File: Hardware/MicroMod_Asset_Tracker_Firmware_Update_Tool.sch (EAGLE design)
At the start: 23 parts, among them J5 MICROMOD-2222, U2 CH340C

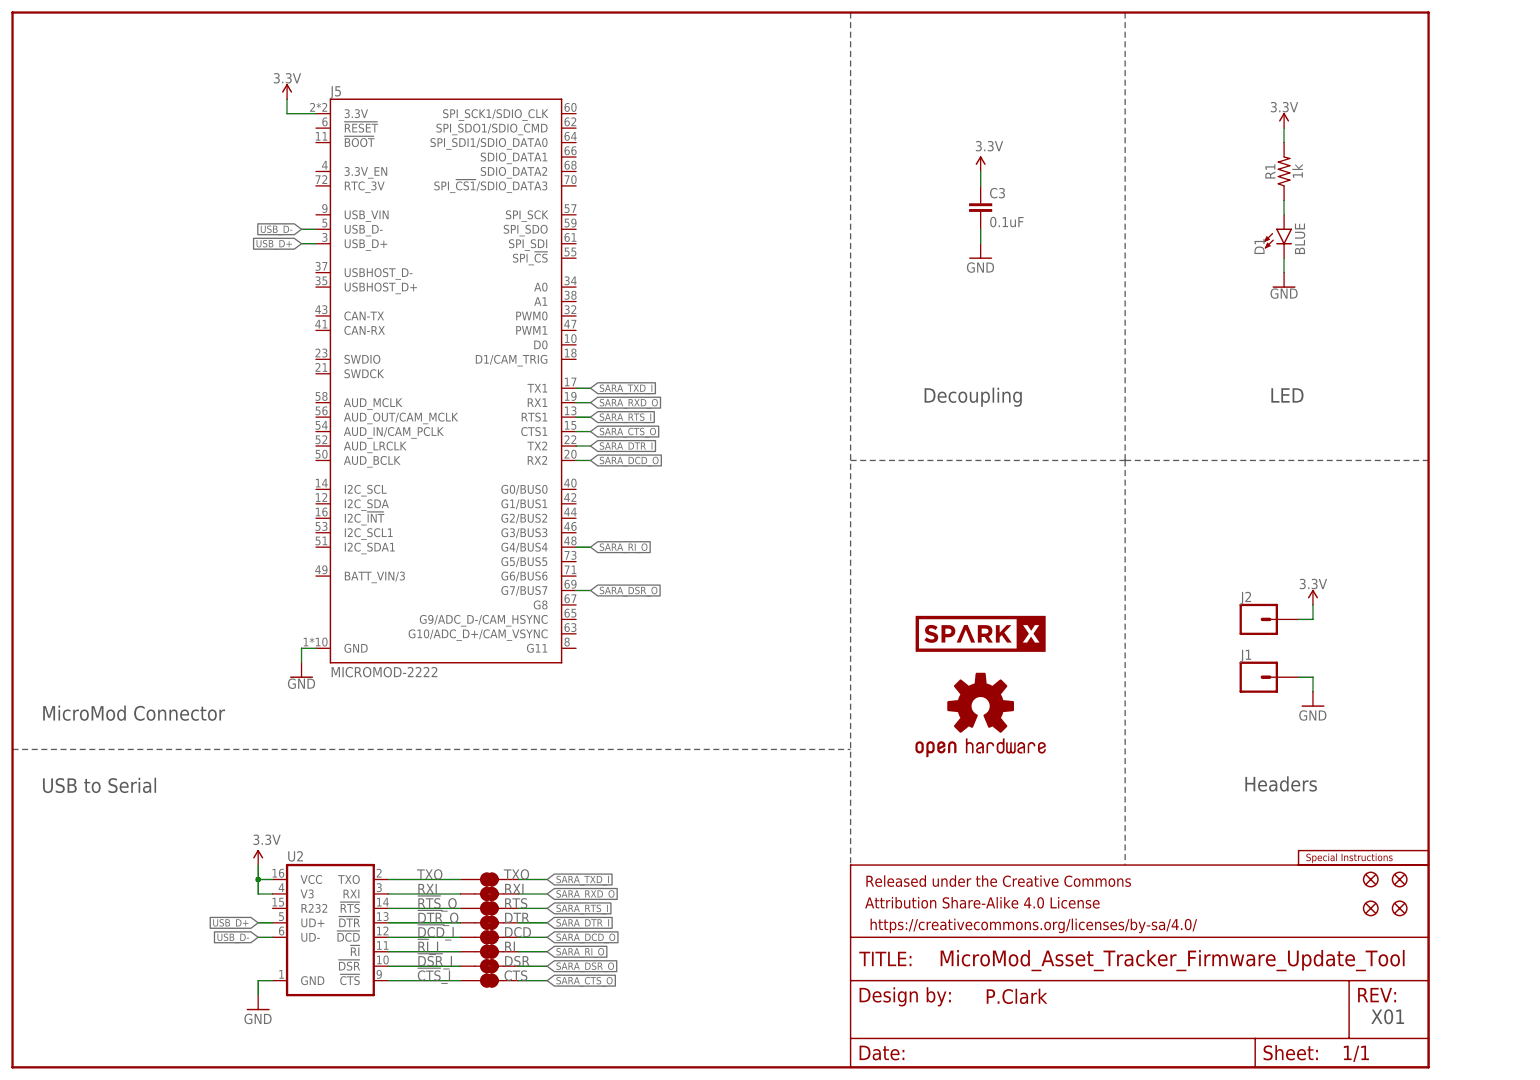
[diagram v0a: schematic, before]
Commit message: Updates for v10
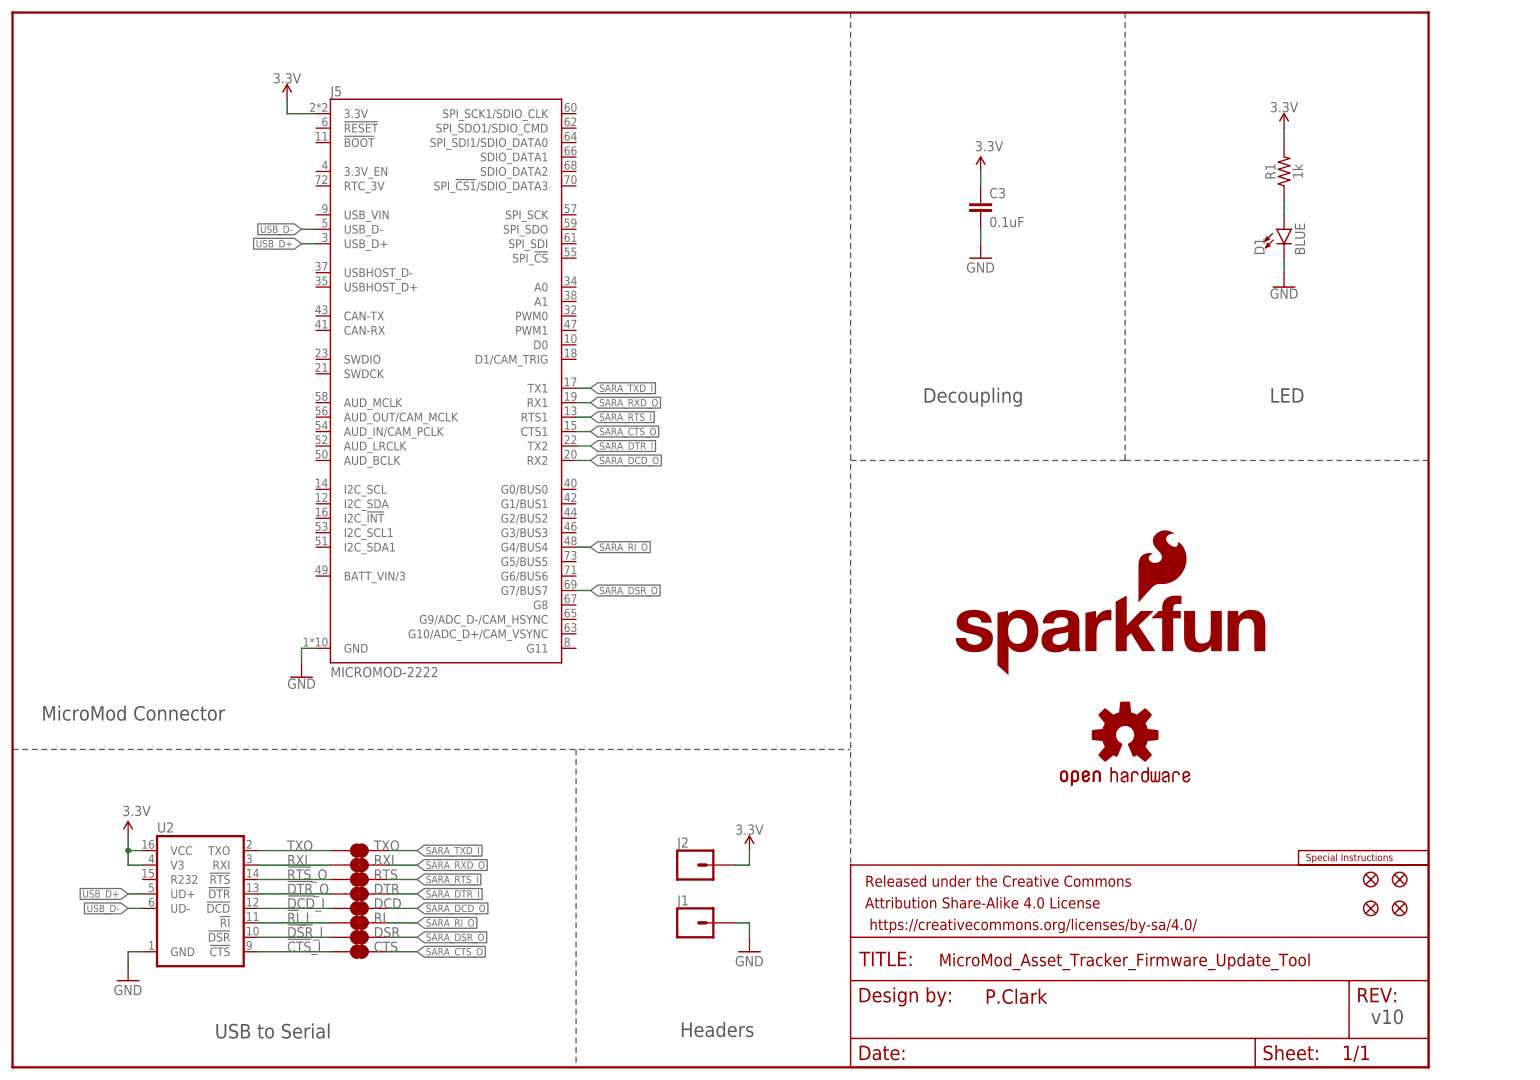
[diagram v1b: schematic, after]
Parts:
- removed SPARKX2: SPARKX-LOGO4, SparkX:SPARKX-LOGO4
- added LOGO3: SFE_LOGO_NAME_FLAME.1_INCH, SparkFun-Aesthetics:SFE_LOGO_NAME_FLAME.1_INCH
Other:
- note added: "v10"
- note removed: "X01"
- moved on the sheet: CTS, DCD, DSR, DTR, J1, J2, RI, RTS, RXI, TXO, U2
